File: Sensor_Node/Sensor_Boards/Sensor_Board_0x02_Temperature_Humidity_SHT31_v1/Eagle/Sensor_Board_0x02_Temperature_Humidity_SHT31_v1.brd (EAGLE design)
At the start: 55 x 35 mm, 16 parts, among them J1 M04_SMD_90, J4 ARDUINO_ISP, U2 ATMEGA328P_TQFP, Y1 8MHZ

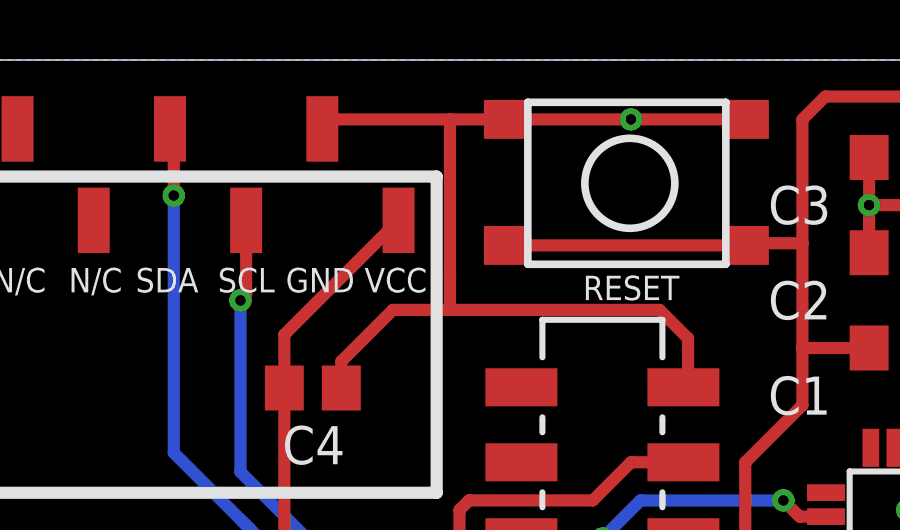
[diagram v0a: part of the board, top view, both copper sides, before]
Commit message: Updated Prototyping Board & DS18B20 Board
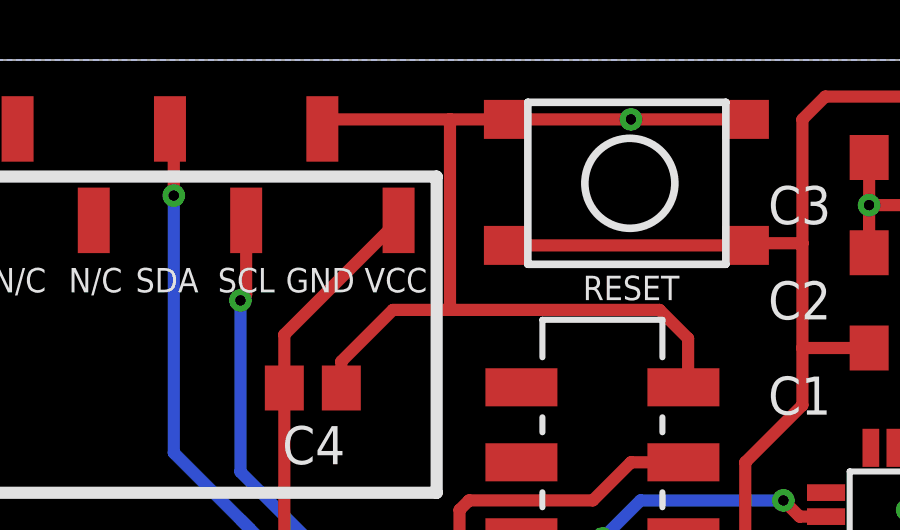
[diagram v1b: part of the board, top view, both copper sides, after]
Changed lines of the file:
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@@
 <?xml version="1.0" encoding="utf-8"?>
 <!DOCTYPE eagle SYSTEM "eagle.dtd">
-<eagle version="8.4.2">
+<eagle version="8.4.3">
 <drawing>
 <settings>
@@
 <wire x1="35.8775" y1="28.5775" x2="35.88" y2="28.575" width="0.4064" layer="1"/>
 <wire x1="35.8775" y1="30.1625" x2="39.6875" y2="30.1625" width="0.4064" layer="1"/>
-<wire x1="21.9075" y1="27.6885" x2="21.9075" y2="27.94" width="0.4064" layer="1"/>
-<wire x1="21.9075" y1="27.94" x2="21.9075" y2="33.02" width="0.4064" layer="1"/>
+<wire x1="21.9075" y1="26.67" x2="21.9075" y2="33.02" width="0.4064" layer="1"/>
 <wire x1="29.845" y1="25.7175" x2="28.8925" y2="26.67" width="0.4064" layer="1"/>
 <wire x1="29.845" y1="25.7175" x2="29.845" y2="24.2475" width="0.4064" layer="1"/>
@@
 <wire x1="21.9075" y1="26.67" x2="28.8925" y2="26.67" width="0.4064" layer="1"/>
 <wire x1="21.9075" y1="26.67" x2="20.0025" y2="26.67" width="0.4064" layer="1"/>
-<wire x1="21.9075" y1="27.94" x2="21.9075" y2="26.67" width="0.4064" layer="1"/>
 </signal>
 <signal name="VCC" class="1">
